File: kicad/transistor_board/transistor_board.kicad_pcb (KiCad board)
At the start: 2 copper layers, 25.4 x 38.1 mm, 16 parts, among them J1 Conn_01x10, J2 Conn_01x02, Q1 MMBF170, Q2 MMBF170, Q3 MMBF170, Q4 MMBF170, U2 ESP32-cam, U3 LM7805_TO220

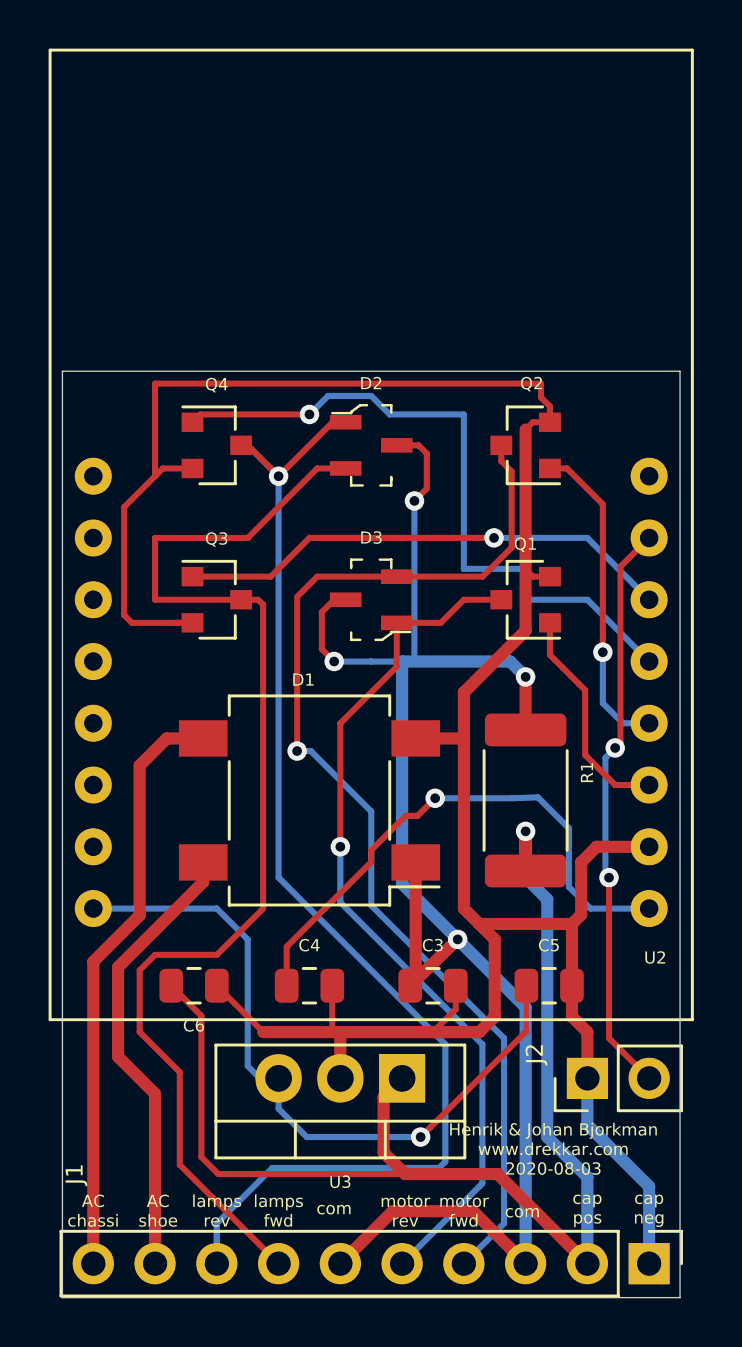
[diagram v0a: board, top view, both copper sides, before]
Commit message: gerber files
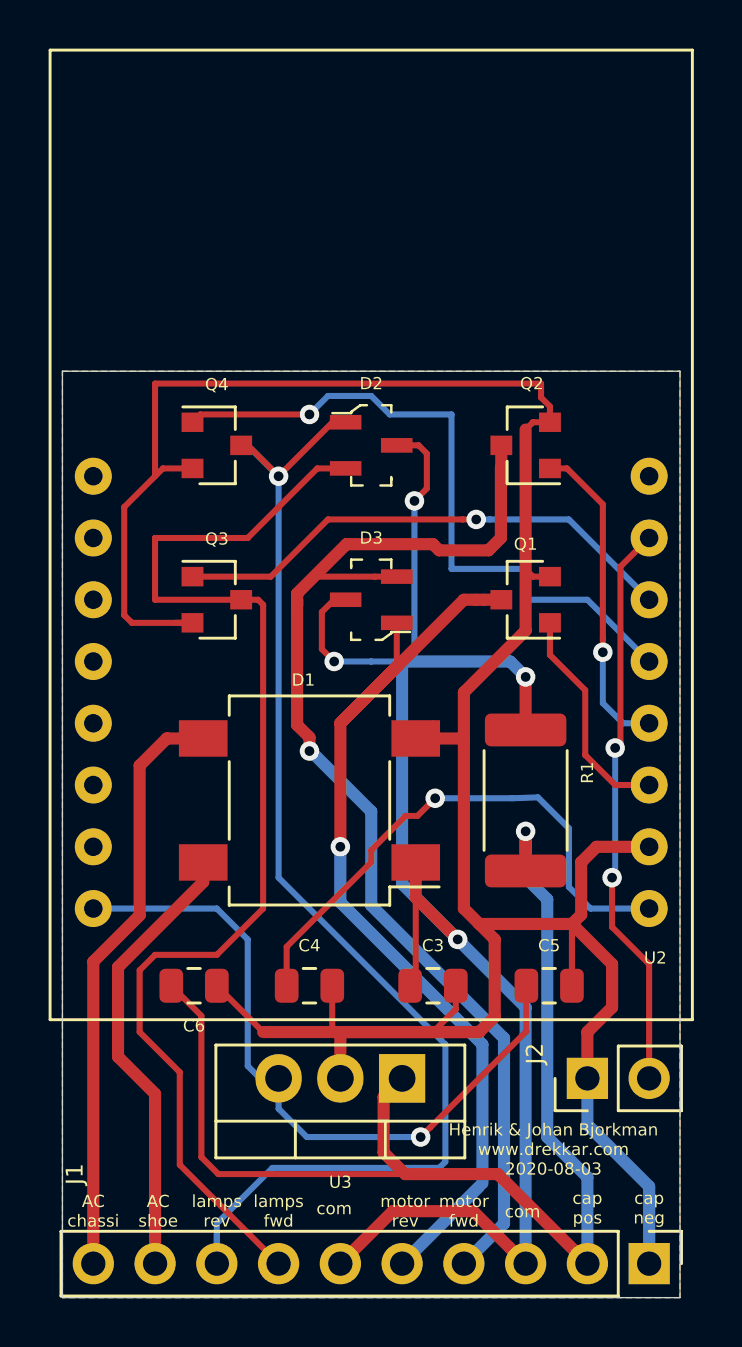
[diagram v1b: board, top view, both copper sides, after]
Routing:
- net Net-(D3-Pad1): track 35.8 -> 39.8 mm
- net GND: track 121.2 -> 124.6 mm
- net Net-(D3-Pad2): track 45.9 -> 48.7 mm
- net Net-(C3-Pad1): track 70.7 -> 71.9 mm
- net Net-(Q3-Pad1): track 20.5 -> 21.1 mm
- added copper zone on F.Cu, net GND
- added copper zone on B.Cu, net Net-(C3-Pad1)
